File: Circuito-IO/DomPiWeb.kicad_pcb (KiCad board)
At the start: 2 copper layers, 108 x 65 mm, 120 parts, among them J1 CONUFL001-SMD-T (Linx), J10 Bx3, J11 Salida 5v, J12 Bateria 12v, J13 12v CA, J2 Salida 5v, J3 SIM7050-6-0-00-A, J4 RaspberryPi GPIO, J5 SIMDBG, J6 EXP1, J7 Bx2, J8 Bx3, J9 Bx2, Q1 DMG2305UXQ6, Q2 DMG2305UXQ6, U1 SIM900, U2 LM2596S-ADJ, U3 LM2596S-ADJ, U4 LM2596S-ADJ, U5 LM2596S-ADJ

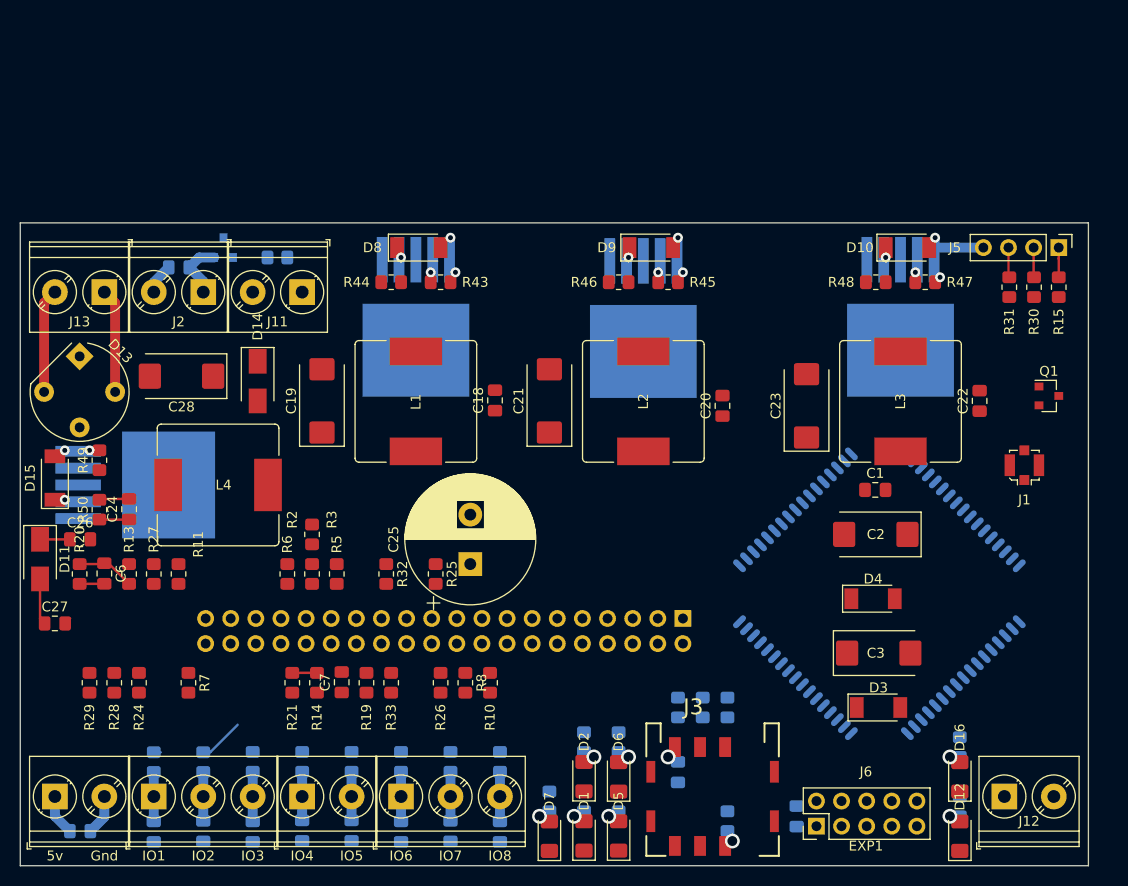
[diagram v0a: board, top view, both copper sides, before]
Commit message: Correccion
Correcciones por rotura y desincronización del repositorio
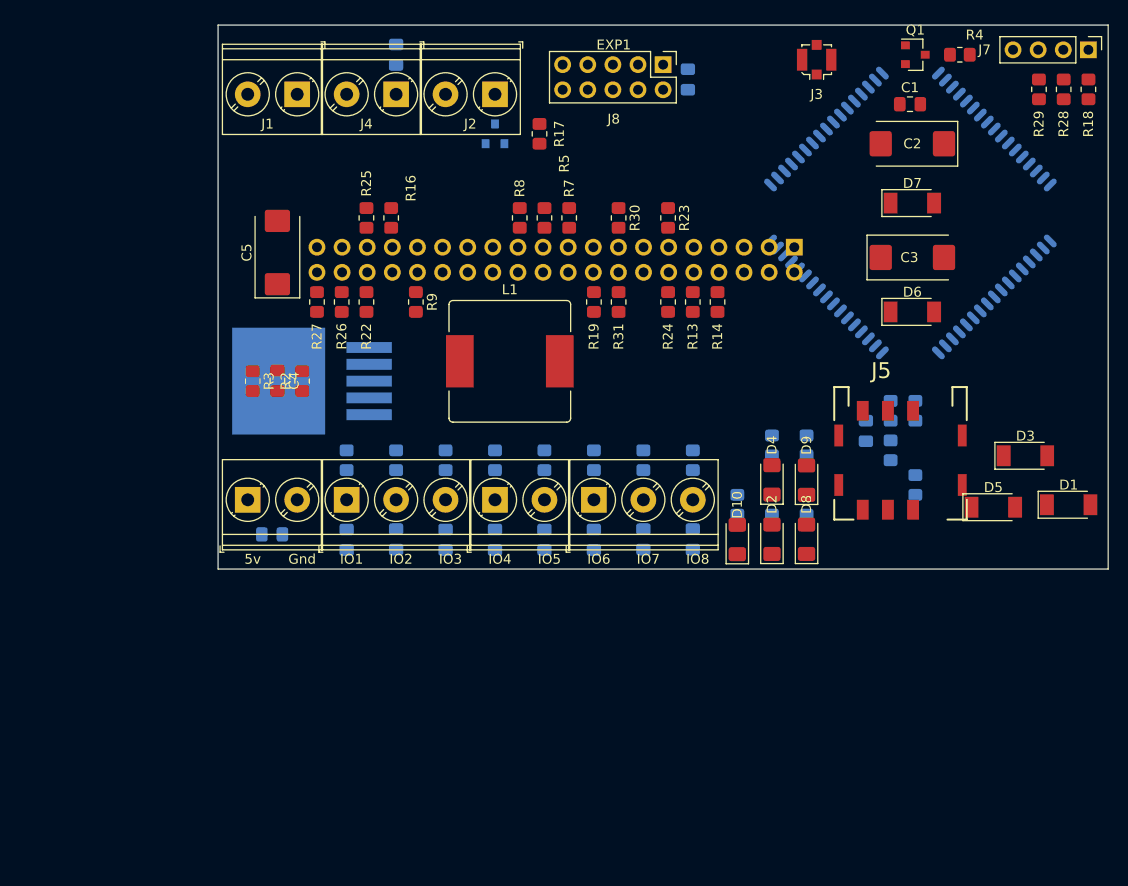
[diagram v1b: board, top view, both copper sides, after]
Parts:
- removed C18, C20, C22, C26, C27: 100nf, Capacitor_SMD:C_0805_2012Metric_Pad1.18x1.45mm_HandSolder
- removed C19, C21, C23, C28: 470uf, Capacitor_Tantalum_SMD:CP_EIA-7343-43_Kemet-X_Pad2.25x2.55mm_HandSolder
- removed C24: 33nf, Capacitor_SMD:C_0805_2012Metric_Pad1.18x1.45mm_HandSolder
- removed C25: 470uf / 25v, Capacitor_THT:CP_Radial_D13.0mm_P5.00mm
- removed the C6 at (78.5, 120.5)
- removed the C7 at (102.5, 131.4)
- removed the D10 at (159.7, 87.5)
- removed D11, D14: M7, Diode_SMD:D_SMA
- removed D12, D16: Led SMD, LED_SMD:LED_1206_3216Metric_Pad1.42x1.75mm_HandSolder
- removed D13: W10G, Diode_THT:Diode_Bridge_Round_D9.8mm
- removed D15: PMEG4050EP, Diode_SMD:D_SOD-128
- removed the D8 at (110.3, 87.5)
- removed the D9 at (133.8, 87.5)
- removed the J11 at (98.5, 92.0)
- removed the J12 at (169.5, 143.0)
- removed J13: 12v CA, TerminalBlock_Phoenix:TerminalBlock_Phoenix_PT-1,5-2-5.0-H_1x02_P5.00mm_Horizontal
- removed the J7 at (73.5, 143.0)
- removed L2, L3, L4: 47uH - SRR1210-470M, Inductor_SMD:L_Bourns_SRR1210A
- removed the R13 at (81.0, 120.5)
- removed the R14 at (100.0, 131.5)
- removed the R20 at (76.0, 120.5)
- removed the R21 at (97.5, 131.5)
- removed R43, R45, R47, R49, R51, R52: 1K, Resistor_SMD:R_0805_2012Metric_Pad1.20x1.40mm_HandSolder
- removed R44, R46: 3K3, Resistor_SMD:R_0805_2012Metric_Pad1.20x1.40mm_HandSolder
- removed R48: 2K2, Resistor_SMD:R_0805_2012Metric_Pad1.20x1.40mm_HandSolder
- removed R50: 10K, Resistor_SMD:R_0805_2012Metric_Pad1.20x1.40mm_HandSolder
- removed U3, U4, U5: LM2596S-ADJ, Package_TO_SOT_SMD:TO-263-5_TabPin3
- added C4: 100nf, Capacitor_SMD:C_0805_2012Metric_Pad1.18x1.45mm_HandSolder, F.Cu at (96.0, 101.0)
- added C5: 470uf, Capacitor_Tantalum_SMD:CP_EIA-7343-43_Kemet-X_Pad2.25x2.55mm_HandSolder, F.Cu at (96.0, 88.0)
- added D1: M7, Diode_SMD:D_SOD-128, F.Cu at (176.0, 113.5)
- added D3: M7, Diode_SMD:D_SOD-128, F.Cu at (171.6, 108.5)
- added D5: PMEG4050EP, Diode_SMD:D_SOD-128, F.Cu at (168.4, 113.8)
- added J1: Entrada 12v, TerminalBlock_Phoenix:TerminalBlock_Phoenix_PT-1,5-2-5.0-H_1x02_P5.00mm_Horizontal, F.Cu at (98.0, 72.0)
- added J2: Salida 5v, TerminalBlock_Phoenix:TerminalBlock_Phoenix_PT-1,5-2-5.0-H_1x02_P5.00mm_Horizontal, F.Cu at (118.0, 72.0)
- added J9: Bx2, TerminalBlock_Phoenix:TerminalBlock_Phoenix_PT-1,5-2-5.0-H_1x02_P5.00mm_Horizontal, F.Cu at (93.0, 113.0)
- added R2: 1K, Resistor_SMD:R_0805_2012Metric_Pad1.20x1.40mm_HandSolder, F.Cu at (98.5, 101.0)
- added R3: 3K3, Resistor_SMD:R_0805_2012Metric_Pad1.20x1.40mm_HandSolder, F.Cu at (93.5, 101.0)
- J4: renamed from J2; value Salida 5v -> Salida 5v Controlada
- R17: renamed from R12; moved to F.Cu
- U1: value SIM900 -> LM2596S-ADJ; footprint RF_GSM:SIMCom_SIM900 -> Package_TO_SOT_SMD:TO-263-5_TabPin3
- U2: value LM2596S-ADJ -> SIM900; footprint Package_TO_SOT_SMD:TO-263-5_TabPin3 -> RF_GSM:SIMCom_SIM900
- moved R4 81.5 mm to (165.0, 68.0), turned to 0 degrees
- moved J8 78.5 mm to (135.0, 69.0), turned to 270 degrees
- moved C8 75.3 mm to (137.5, 70.5), turned to 270 degrees
- moved U1 61.3 mm to (99.5, 101.0), turned to 180 degrees
- moved U2 51.1 mm to (160.0, 84.0), turned to 135 degrees
- moved J3 46.1 mm to (150.5, 68.5)
- moved R13 44.8 mm to (138.0, 93.0)
- moved R14 44.8 mm to (140.5, 93.0)
- moved R19 44.8 mm to (128.0, 93.0)
- moved R22 44.8 mm to (105.0, 93.0)
- moved R24 44.8 mm to (135.5, 93.0)
- moved R26 44.8 mm to (102.5, 93.0)
- moved R27 44.8 mm to (100.0, 93.0)
- moved R31 44.8 mm to (130.5, 93.0)
- moved R9 44.8 mm to (110.0, 93.0)
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- renumbered C4 to C6, C5 to C7, D7 to D10, D1 to D2, D2 to D4, D3 to D6, D4 to D7, D5 to D8, D6 to D9, J8 to J10, J9 to J11, J10 to J12, J1 to J3, J3 to J5, J4 to J6, J5 to J7, J6 to J8, R16 to R10, R17 to R11, R18 to R12, R8 to R13, R10 to R14, R9 to R15, R11 to R16, R15 to R18, R22 to R20, R23 to R21, R24 to R22, R25 to R23, R26 to R24, R27 to R25, R28 to R26, R29 to R27, R30 to R28, R31 to R29, R32 to R30, R33 to R31, R34 to R32, R35 to R33, R36 to R34, R37 to R35, R38 to R36, R39 to R37, R40 to R38, R41 to R39, R2 to R4, R42 to R40, R3 to R5, R4 to R6, R5 to R7, R6 to R8, R7 to R9
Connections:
- net +4V renamed Net-(D1-Pad1)
- C7 pad 1: Net-(C5-Pad1) -> Net-(C7-Pad1)
- D6 pad 2: Net-(D3-Pad2) -> Net-(D6-Pad2)
- D7 pad 2: Net-(D4-Pad2) (its old number) -> Net-(D7-Pad2)
- J3 pad 1: Net-(J1-Pad1) -> Net-(J3-Pad1)
- J5 pad C1: Net-(C5-Pad1) -> Net-(C7-Pad1)
- L1 pad 1: Net-(D8-Pad1) -> Net-(D5-Pad1)
- R10 pad 2: Net-(R16-Pad2) -> Net-(R10-Pad2)
- R11 pad 2: Net-(R17-Pad2) -> Net-(R11-Pad2)
- R12 pad 2: Net-(R18-Pad2) -> Net-(R12-Pad2)
- R13 pad 2: Net-(R8-Pad2) -> Net-(R13-Pad2)
- R14 pad 2: Net-(R10-Pad2) -> Net-(R14-Pad2)
- R15 pad 2: Net-(C5-Pad1) -> Net-(C7-Pad1)
- R20 pad 1: Net-(R22-Pad1) -> Net-(R20-Pad1)
- R21 pad 1: Net-(R23-Pad1) -> Net-(R21-Pad1)
- R28 pad 2: Net-(R30-Pad2) -> Net-(R28-Pad2)
- R29 pad 2: Net-(R31-Pad2) -> Net-(R29-Pad2)
- R6 pad 1: Net-(R4-Pad1) -> Net-(R6-Pad1)
- R7 pad 2: Net-(R4-Pad1) -> Net-(R6-Pad1)
- R9 pad 2: Net-(R7-Pad2) -> Net-(R9-Pad2)
- U1 pad 1: Net-(D4-Pad2) (its old number) -> Net-(D3-Pad1)
- U1 pad 2: Net-(U1-Pad2) -> Net-(D5-Pad1)
- U1 pad 4: Net-(R7-Pad2) -> Net-(R2-Pad1)
- U1 pad 5: Net-(U1-Pad5) -> GND
- U2 pad 1: Net-(C25-Pad1) -> Net-(D7-Pad2)
- U2 pad 2: Net-(D8-Pad1) -> Net-(U2-Pad2)
- U2 pad 4: Net-(R43-Pad1) -> Net-(R9-Pad2)
- U2 pad 5: GND -> Net-(U2-Pad5)
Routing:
- net GND: track 15.3 -> 0.00 mm, vias 6 -> 0
- net Net-(D13-Pad4): track 10.5 -> 0.00 mm
- net Net-(D13-Pad2): track 10.5 -> 0.00 mm
- net VBatSense: track 7.70 -> 0.00 mm
- net Net-(C6-Pad1): track 6.01 -> 0.00 mm
- net Net-(J6-Pad37): track 5.83 -> 0.00 mm
- net Net-(C15-Pad1): track 5.01 -> 0.00 mm
- net Net-(C12-Pad1): track 5.01 -> 0.00 mm
- net Net-(C10-Pad1): track 5.01 -> 0.00 mm
- net Net-(C17-Pad1): track 4.99 -> 0.00 mm
- net Net-(C11-Pad1): track 4.96 -> 0.00 mm
- net Net-(C16-Pad1): track 4.94 -> 0.00 mm
- net Net-(C14-Pad1): track 4.91 -> 0.00 mm
- net Net-(C13-Pad1): track 4.91 -> 0.00 mm
- net Net-(J6-Pad28): track 4.63 -> 0.00 mm
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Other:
- board size 108 x 65 mm -> 90 x 55 mm
